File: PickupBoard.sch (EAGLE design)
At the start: 21 parts, among them IC2 TL072

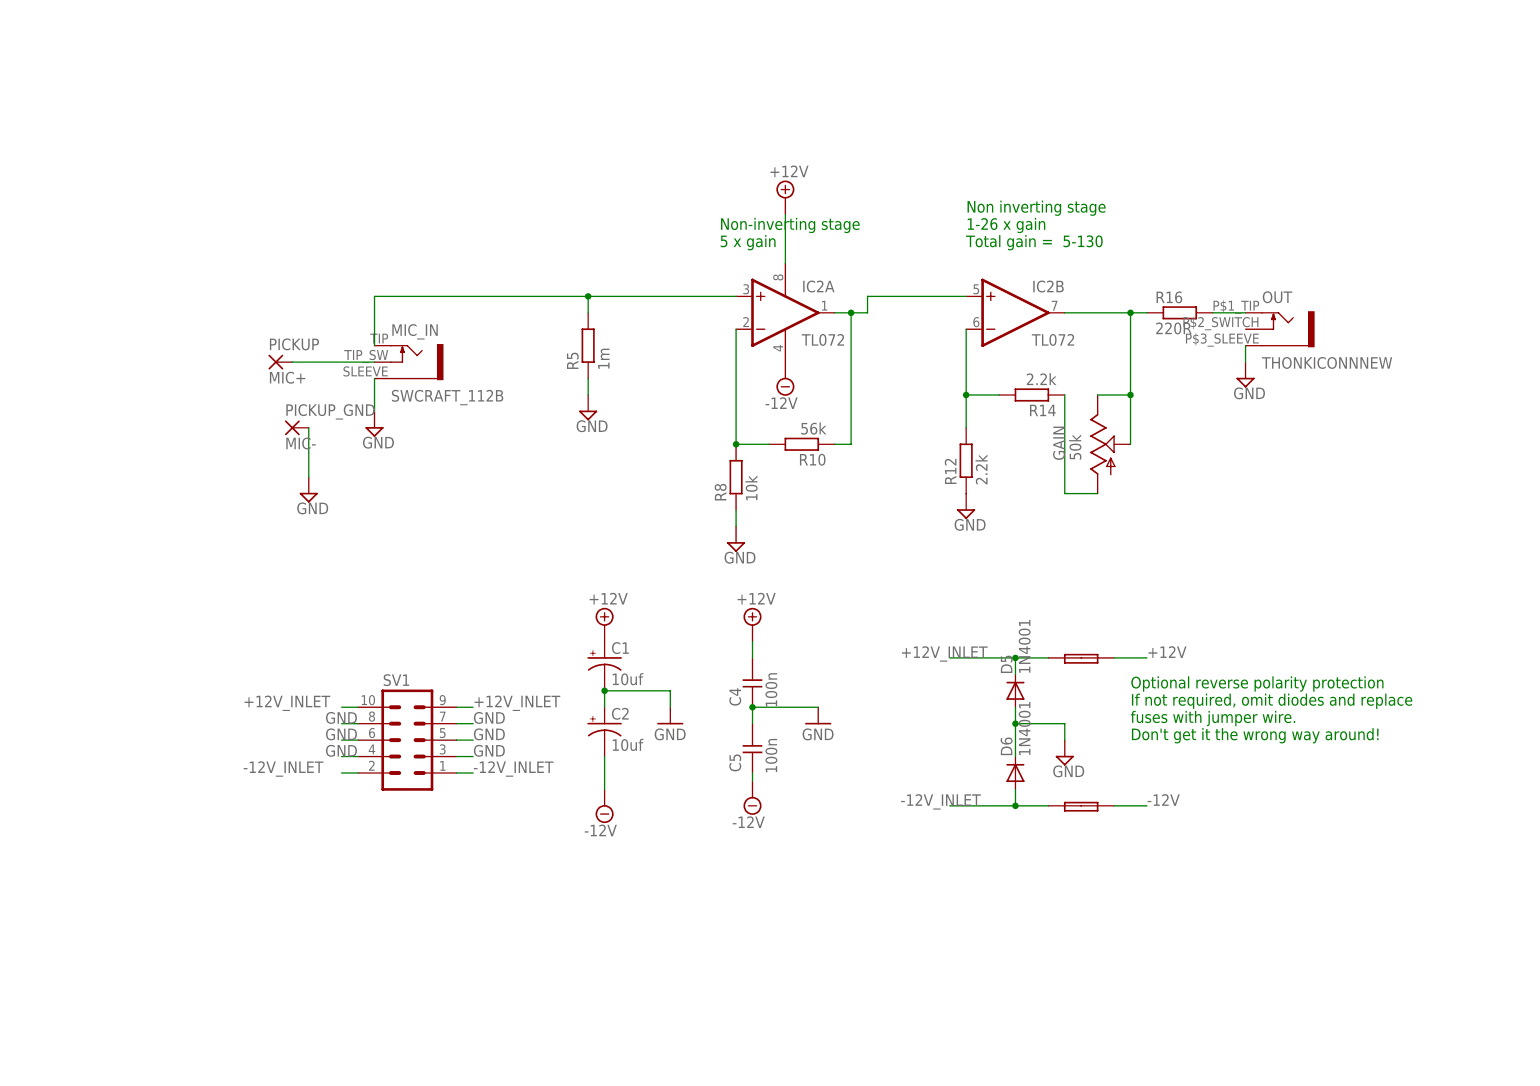
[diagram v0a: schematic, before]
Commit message: Building the circuit
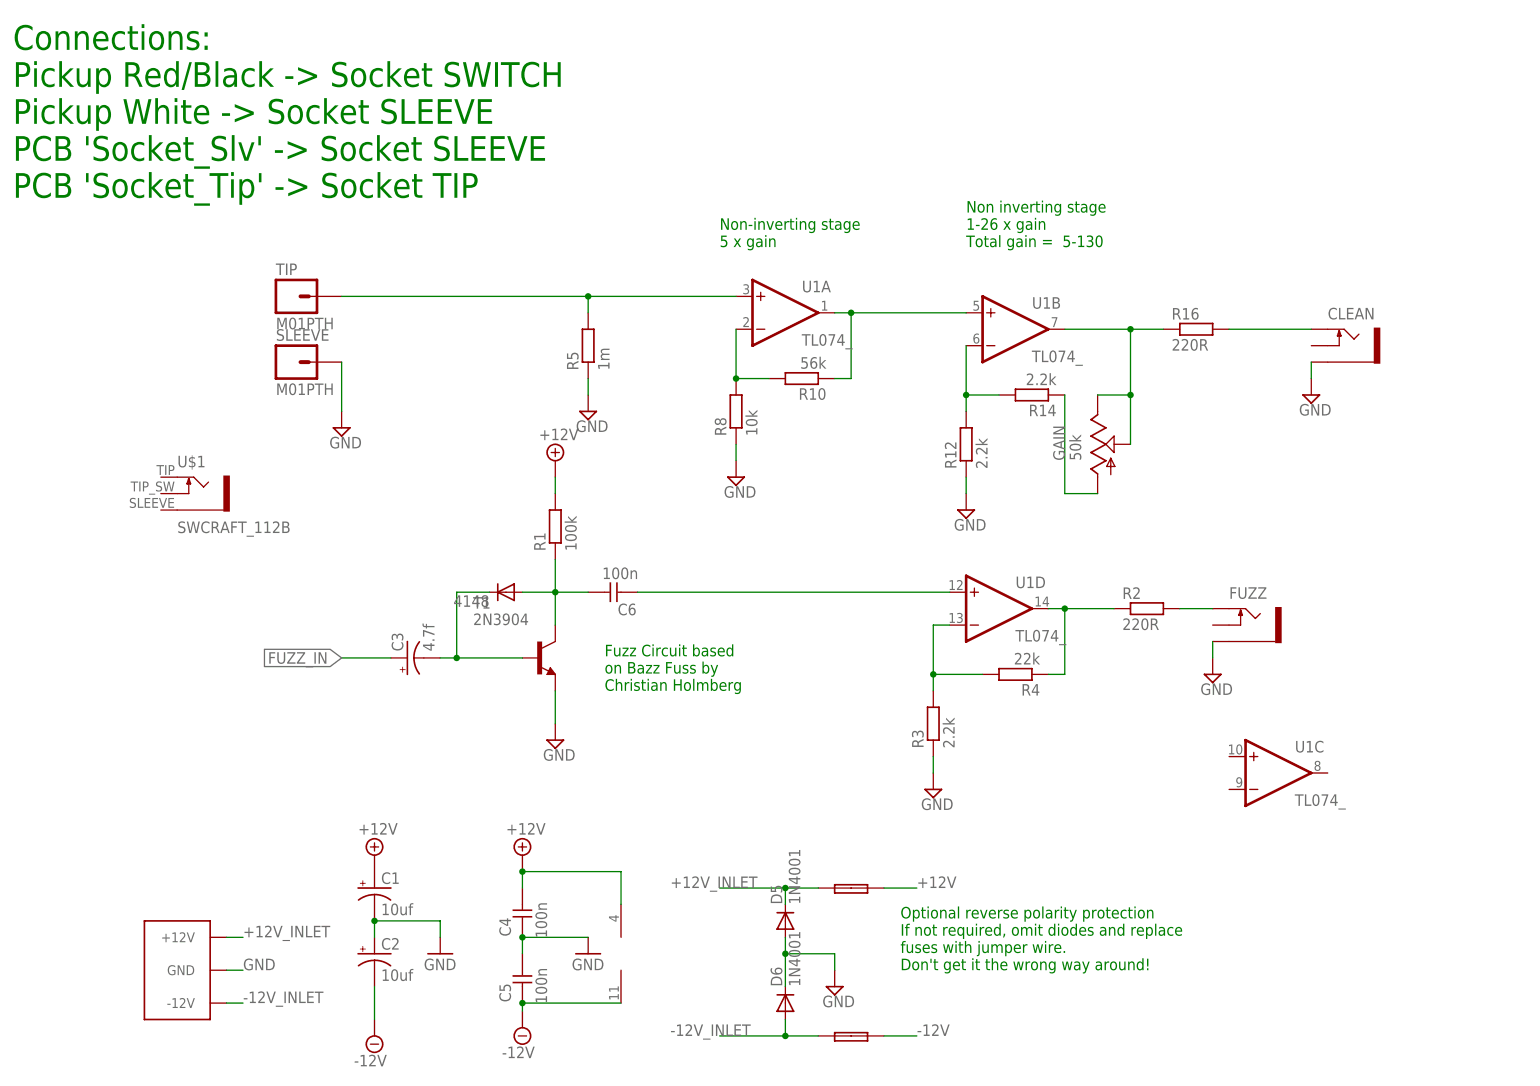
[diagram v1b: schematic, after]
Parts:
- removed IC2: TL072, TomW:TL072P
- removed MIC_IN: SWCRAFT_112B, TomW:SWCRAFT_112B
- removed OUT: THONKICONNNEW, MusicThingModular:THONKICONNNEW
- removed PICKUP: MIC+, TomW:LONG_PAD_1
- removed PICKUP_GND: MIC-, TomW:LONG_PAD_1
- removed SV1: (no value), TomW:10_PIN_HEADER
- added 4148: (no value), MusicThingModular:SMALL_DIODEDO35-7
- added C3: 4.7f, SparkFun-Passives:CAP_POLPTH2
- added C6: 100n, TomW:C-EU050-024X044
- added CLEAN, FUZZ: THONKICONNNEW, MusicThingModular:THONKICONNNEW
- added R1: 100k, MusicThingModular:RESISTOR7MM
- added R2: 220R, MusicThingModular:RESISTOR7MM
- added R3: 2.2k, MusicThingModular:RESISTOR7MM
- added R4: 22k, MusicThingModular:RESISTOR7MM
- added SLEEVE, TIP: M01PTH, SparkFun-Connectors:M01PTH
- added T1: 2N3904, transistor:2N3904
- added U$1: SWCRAFT_112B, TomW:SWCRAFT_112B
- added U$2: EURO_POWER_LOCK, MusicThingModular:EURO_POWER_LOCK
- added U1: TL074_, MusicThingModular:TL074_
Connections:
- new net FUZZ_IN: C3.+
- new net N$11: R3.2, R4.2, U1D.-IN
- new net N$12: R2.1, R4.1, U1D.OUT
- new net N$13: FUZZ.TIP, R2.2
- new net N$7: 4148.C, C3.-, T1.B
- new net N$9: 4148.A, C6.1, R1.1, T1.C
- net +12V: now also R1.2, U1P.V+; no longer IC2P.V+
- net +12V_INLET: now also U$2.+12V; no longer SV1.10, SV1.9
- net -12V: now also U1P.V-; no longer IC2P.V-
- net -12V_INLET: now also U$2.-12V; no longer SV1.1, SV1.2
- net GND: now also CLEAN.SLEEVE, FUZZ.SLEEVE, R3.1, SLEEVE.1, T1.E, U$2.GND; no longer MIC_IN.5, OUT.SLEEVE, PICKUP_GND.P, SV1.3, SV1.4, SV1.5, SV1.6, SV1.7, SV1.8
- net N$1: now also C6.2, U1D.+IN; no longer MIC_IN.4, PICKUP.P
- net N$10: now also CLEAN.TIP; no longer OUT.TIP
- net N$2: now also TIP.1, U1A.+IN; no longer IC2A.+IN, MIC_IN.3
- net N$3: now also U1A.-IN; no longer IC2A.-IN
- net N$4: now also U1A.OUT, U1B.+IN; no longer IC2A.OUT, IC2B.+IN
- net N$6: now also U1B.-IN; no longer IC2B.-IN
- net N$8: now also U1B.OUT; no longer IC2B.OUT
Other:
- note added: "Connections: Pickup Red/Black -> Socket SWITCH Pickup White -> Socket SLEEVE PCB 'Socket_Slv' -> Socket SLEEVE PCB 'Socket_Tip' -> Socket TIP"
- note added: "Fuzz Circuit based on Bazz Fuss by Christian Holmberg"
- moved on the sheet: C1, C2, C4, C5, D5, D6, R10, R12, R16, R8
